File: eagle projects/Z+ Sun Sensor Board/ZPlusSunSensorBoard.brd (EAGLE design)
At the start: 78 x 78 mm, 51 parts, among them U2 ADS7841E_2K5, U4 LM20BIM7X_NOPB, U6 TLV9051IDCKR, U8 TLV9051IDCKR, U9 TLV9051IDCKR

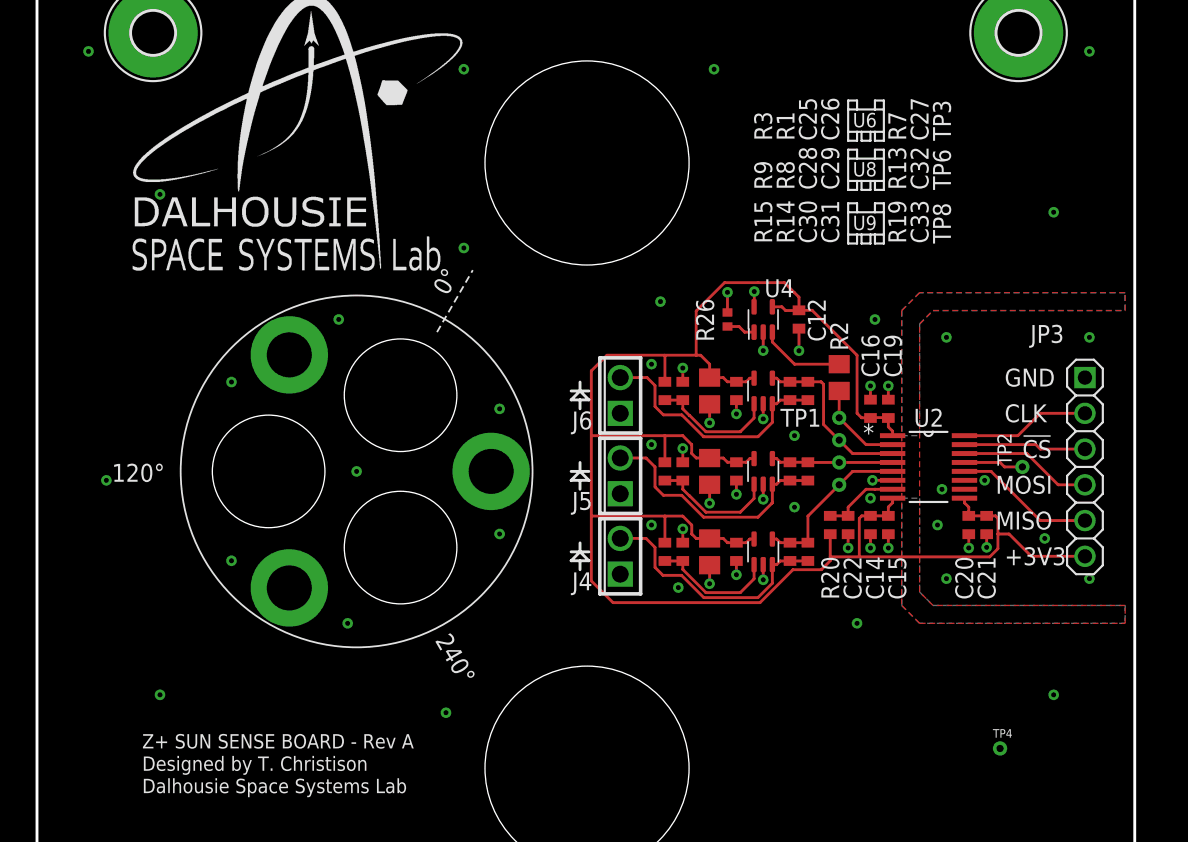
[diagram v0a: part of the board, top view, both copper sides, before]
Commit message: Rev B almost ready
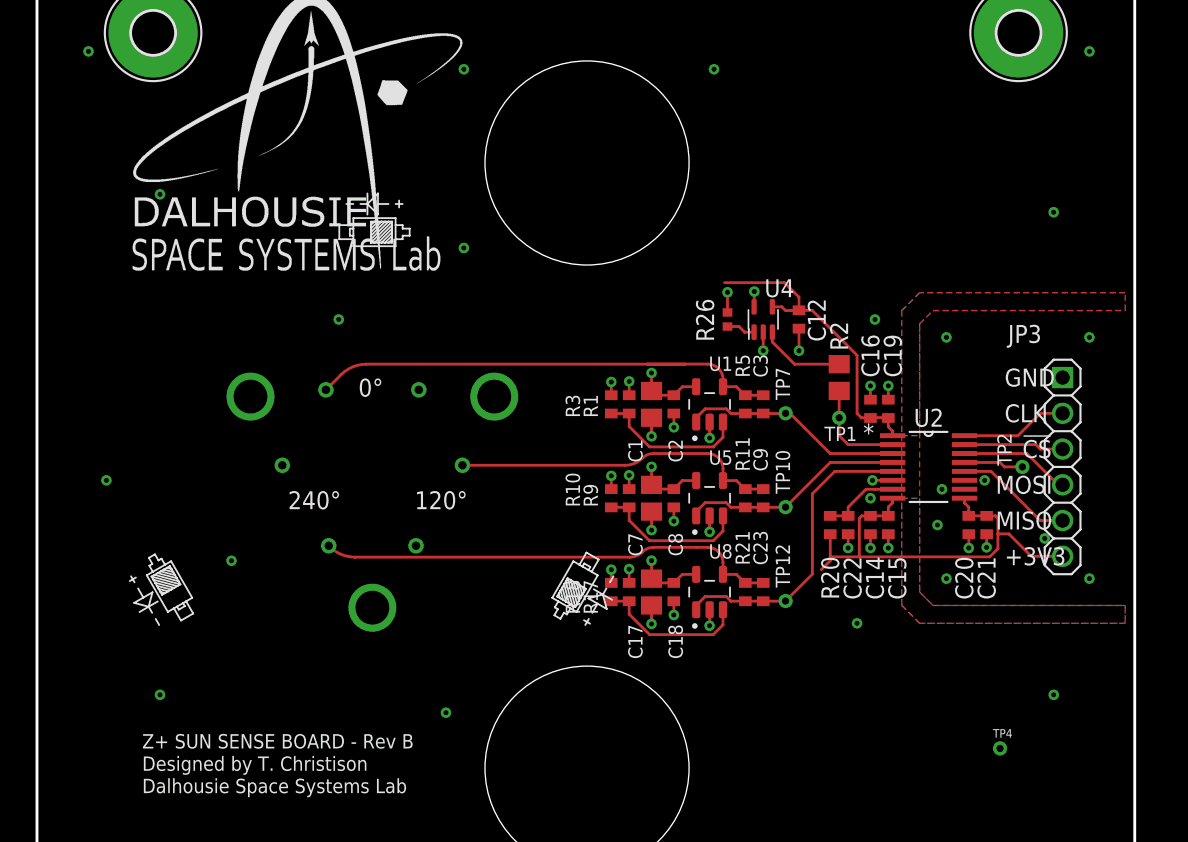
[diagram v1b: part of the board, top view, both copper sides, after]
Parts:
- removed A1: SUN_SENSOR_MOUNT, my_library:SUN_SENOR_MASK
- removed C25, C28, C30: 4.7u, rcl:C0805
- removed C26, C29, C31: 0.1u, resistor:C0402
- removed C27, C32, C33: 0.022u, resistor:C0402
- removed DRILEGEND: (no value), drilegend:DRILEGEND
- removed J4, J5, J6: (no value), my_library:2POL254
- removed R13, R19, R7: 3.74k, resistor:R0402
- removed R14, R8: 280R, resistor:R0402
- removed R15: 13.7k, resistor:R0402
- removed TP3, TP6, TP8: TESTPOINT, my_library:TP_P76H50
- removed U6, U9: TLV9051IDCKR, my_library:SC70-5P65_210X110L36X22N_TLV9051
- added C1, C17, C7: 4.7u, rcl:C0805
- added C18, C2, C8: 0.1u, resistor:C0402
- added C23, C3, C9: 0.022u, resistor:C0402
- added R10, R18: 13.7k, resistor:R0402
- added R11, R21, R5: 3.74k, resistor:R0402
- added R17: 280R, resistor:R0402
- added TP10, TP12, TP7: TESTPOINT, my_library:TP_P76H50
- added U$1: SSR_MOUNT_03, my_library:SSR_MOUNT_03
- added U$2, U$3, U$4: (no value), my_library:PHOTODIODE_SILK
- added U1, U5: TSV991AILT, my_library:SOT95P280X145-5N
- R9: value 13.7k -> 280R
- U8: value TLV9051IDCKR -> TSV991AILT; device my_library:SC70-5P65_210X110L36X22N_TLV9051 -> my_library:SOT95P280X145-5N
- moved U8 9.38 mm to (54.3, 36.5), turned to 90 degrees
- moved R1 3.93 mm to (48.6, 49.8)
- moved R3 3.93 mm to (47.3, 49.8)
- moved R9 3.18 mm to (48.6, 43.2), turned to 270 degrees
- moved JP3 1.59 mm to (79.4, 45.4)
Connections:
- removed net N$13: R14.2, R15.1, U9.1
- removed net N$6: R1.2, R3.1, U6.1
- removed net N$9: R8.2, R9.1, U8.1
- new net N$11: C9.1, R11.1, U$1.C2, U5.4
- new net N$14: R10.1, R9.2, U5.3
- new net N$20: R17.2, R18.1, U8.3
- net +3V3: now also C1.1, C17.1, C18.1, C2.1, C7.1, C8.1, R10.2, R18.2, U1.5, U5.5; no longer C25.1, C26.1, C28.1, C29.1, C30.1, C31.1, R15.2, R9.2, U6.5, U9.5
- net 0_DEGREES: now also C3.2, R5.2, TP7.1, U1.1; no longer C27.2, R7.2, TP3.1, U6.4
- net 120_DEGREES: now also C9.2, R11.2, TP10.1, U5.1; no longer C32.2, R13.2, TP6.1, U8.4
- net 240_DEGREES: now also C23.2, R21.2, TP12.1, U8.1; no longer C33.2, R19.2, TP8.1, U9.4
- net GND: now also C1.2, C17.2, C18.2, C2.2, C7.2, C8.2, R17.1, R9.1, U$1.A1, U$1.A2, U$1.A3, U1.2, U5.2; no longer C25.2, C26.2, C28.2, C29.2, C30.2, C31.2, J4.1, J5.1, J6.1, R14.1, R8.1, U6.2, U9.2
- net N$12: now also C23.1, R21.1, U$1.C3, U8.4; no longer C33.1, J4.2, R19.1, U9.3
- net N$3: now also C3.1, R5.1, U$1.C1, U1.4; no longer C27.1, J6.2, R7.1, U6.3
- net N$8: now also R1.2, R3.1, U1.3; no longer C32.1, J5.2, R13.1, U8.3
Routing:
- net +3V3: track 139.6 -> 71.6 mm, vias 0 -> 6
- net N$11: track 0.00 -> 23.2 mm
- net N$3: track 17.8 -> 35.7 mm
- net N$12: track 17.8 -> 33.3 mm
- net N$20: track 0.00 -> 11.2 mm
- net N$14: track 0.00 -> 11.2 mm
- net 240_DEGREES: track 11.9 -> 21.8 mm
- net N$9: track 9.05 -> 0.00 mm
- net N$6: track 9.05 -> 0.00 mm
- net N$13: track 9.05 -> 0.00 mm
- net 120_DEGREES: track 8.66 -> 16.0 mm
- net N$8: track 17.8 -> 11.2 mm
- net 0_DEGREES: track 12.4 -> 15.8 mm
- net UCB0_SPI_MOSI: track 9.48 -> 7.89 mm
- net UCB0_SPI_MISO: track 10.0 -> 8.42 mm
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- added copper zone on layer 15, net +3V4
- added copper zone on layer 15, net +3V6
- added copper zone on layer 15, net +3V8
- added copper zone on layer 2, net GND3
- added copper zone on layer 2, net GND5
- added copper zone on layer 2, net GND7
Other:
- board text added: "Z+ SUN SENSE BOARD - Rev B"
- board text removed: "01-16"
- board text removed: "01-20"
- board text removed: "LAYER-STACK"
- board text removed: "U6"
- board text removed: "U8"
- board text removed: "U9"
- board text removed: "Z+ SUN SENSE BOARD - Rev A"
